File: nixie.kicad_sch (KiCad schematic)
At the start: 28 parts, among them IC1 SN74141, IC2 SN74141, IC3 SN74141, IC4 SN74141, IC5 MIC5219-5.0YM5-TR, IC6 DS3231M+TRL, J1 1984989

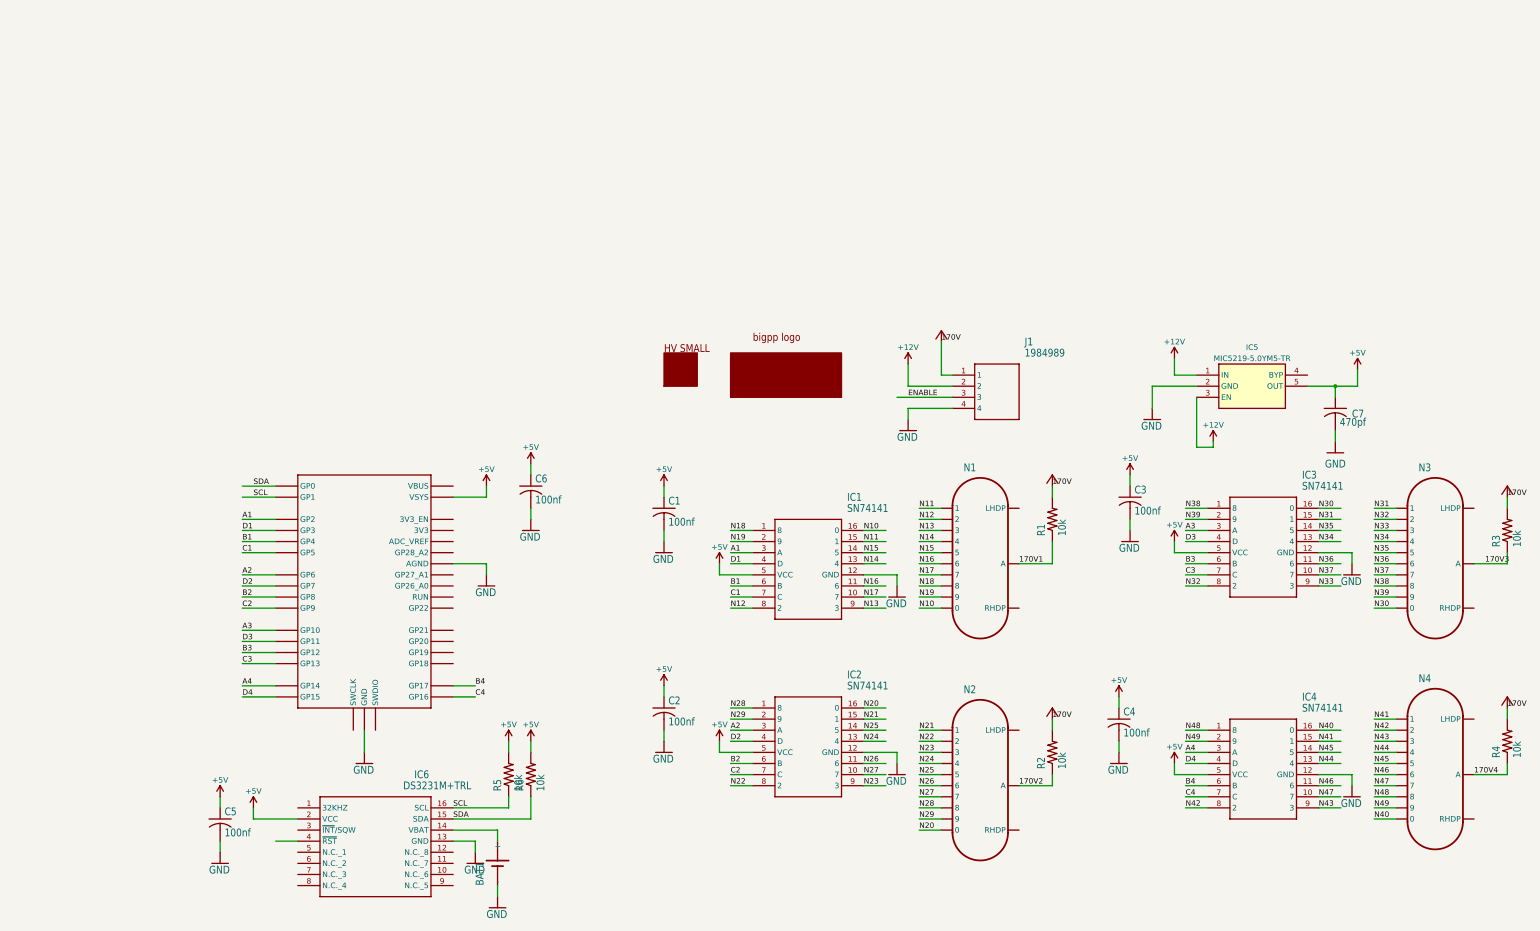
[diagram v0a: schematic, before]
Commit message: Adding WIP files
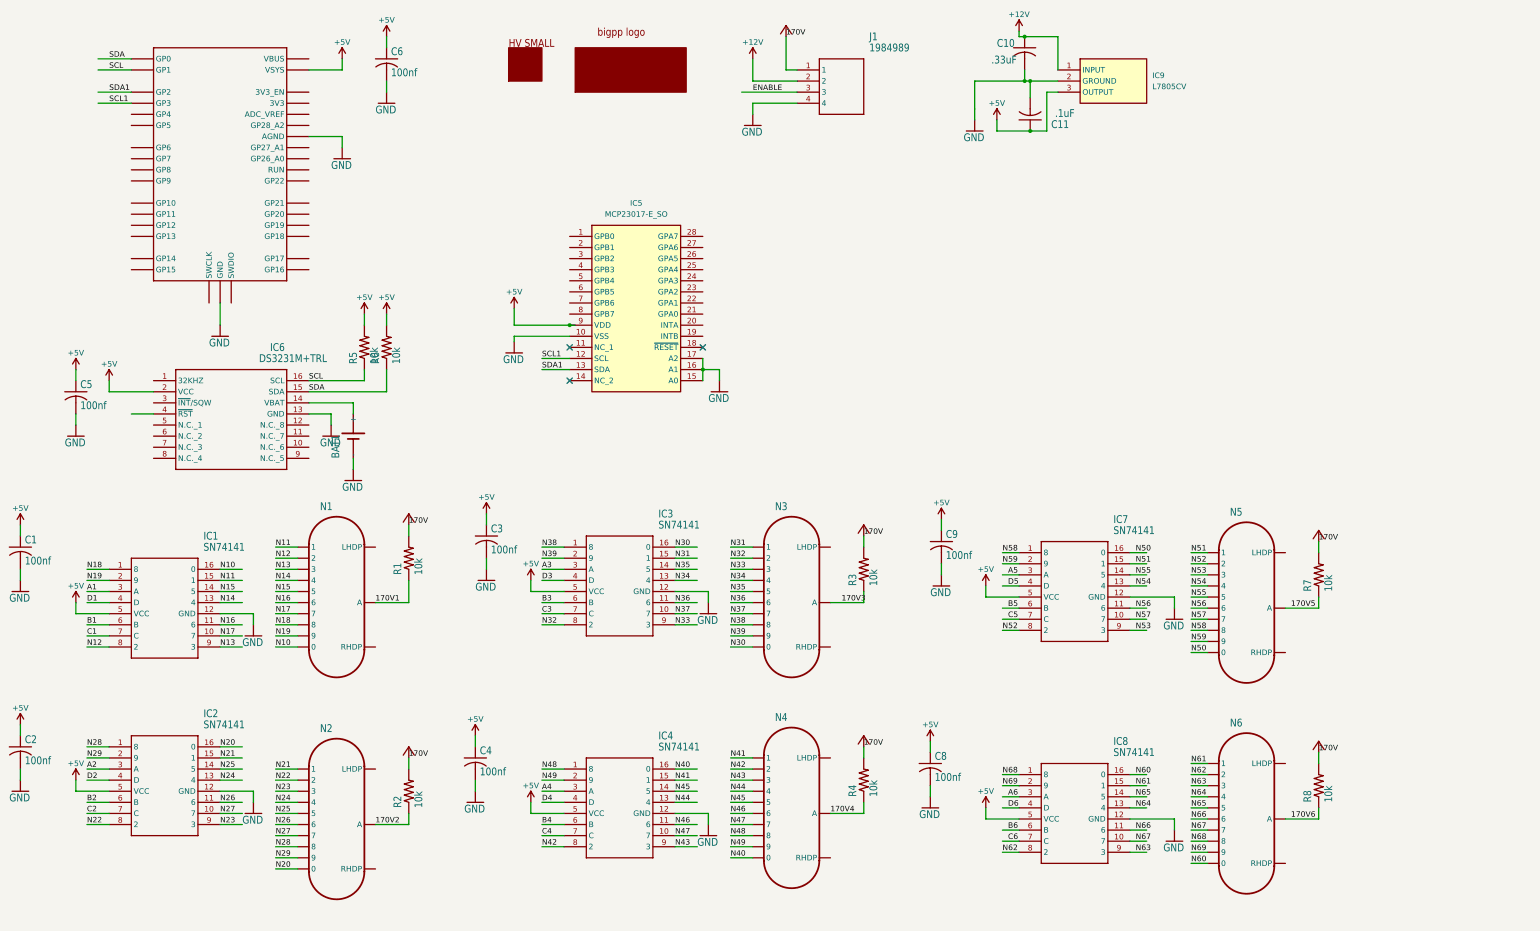
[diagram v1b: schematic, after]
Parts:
- removed C7: 470pf, nixie:C0805, symbol nixie-eagle-import:C-USC0805
- removed IC5: MIC5219-5.0YM5-TR, SOT95P280X130-5N, symbol MIC5219-5_0YM5-TR:MIC5219-5.0YM5-TR
- added C10: .33uF, nixie:C0805, symbol nixie-eagle-import:C-USC0805
- added C11: .1uF, nixie:C0805, symbol nixie-eagle-import:C-USC0805
- added C8, C9: 100nf, nixie:C0805, symbol nixie-eagle-import:C-USC0805
- added IC5: MCP23017-E_SO, L7805CV:SOIC127P1030X265-28N, symbol MCP23017-E_SO:MCP23017-E_SO
- added IC7, IC8: SN74141, TimeExpander:DIP16-2.54-19.2X7.62MM, symbol nixie-eagle-import:SN74141
- added IC9: L7805CV, L7805CV:TO255P460X1020X2008-3P, symbol L7805CV:L7805CV
- added N5, N6: IN-14, nixie:IN-14, symbol nixie-eagle-import:IN-14
- added R7, R8: 10k, nixie:R0805, symbol nixie-eagle-import:R-US_R0805
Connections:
- net +12V: now also C10.1, IC9.1 (INPUT)
- net +5V: now also C11.1, C8.1, C9.1, IC5.9 (VDD), IC7.5 (VCC), IC8.5 (VCC), IC9.3 (OUTPUT)
- net A1: no longer U$1.GP2
- net A2: no longer U$1.GP6
- net A3: no longer U$1.GP10
- net A4: no longer U$1.GP14
- net B1: no longer U$1.GP4
- net B2: no longer U$1.GP8
- net B3: no longer U$1.GP12
- net B4: no longer U$1.GP17
- net C1: no longer U$1.GP5
- net C2: no longer U$1.GP9
- net C3: no longer U$1.GP13
- net C4: no longer U$1.GP16
- net D1: no longer U$1.GP3
- net D2: no longer U$1.GP7
- net D3: no longer U$1.GP11
- net D4: no longer U$1.GP15
- net GND: now also C10.2, C11.2, C8.2, C9.2, IC5.10 (VSS), IC5.15 (A0), IC5.16 (A1), IC5.17 (A2), IC7.12 (GND), IC8.12 (GND), IC9.2 (GROUND)
- net VCC: now also R7.2, R8.2
- new net 170V5: N5.A, R7.1
- new net 170V6: N6.A, R8.1
- new net A5: IC7.3 (A)
- new net A6: IC8.3 (A)
- new net B5: IC7.6 (B)
- new net B6: IC8.6 (B)
- new net C5: IC7.7 (C)
- new net C6: IC8.7 (C)
- new net D5: IC7.4 (D)
- new net D6: IC8.4 (D)
- new net N50: IC7.16 (0), N5.0
- new net N51: IC7.15 (1), N5.1
- new net N52: IC7.8 (2), N5.2
- new net N53: IC7.9 (3), N5.3
- new net N54: IC7.13 (4), N5.4
- new net N55: IC7.14 (5), N5.5
- new net N56: IC7.11 (6), N5.6
- new net N57: IC7.10 (7), N5.7
- new net N58: IC7.1 (8), N5.8
- new net N59: IC7.2 (9), N5.9
- new net N60: IC8.16 (0), N6.0
- new net N61: IC8.15 (1), N6.1
- new net N62: IC8.8 (2), N6.2
- new net N63: IC8.9 (3), N6.3
- new net N64: IC8.13 (4), N6.4
- new net N65: IC8.14 (5), N6.5
- new net N66: IC8.11 (6), N6.6
- new net N67: IC8.10 (7), N6.7
- new net N68: IC8.1 (8), N6.8
- new net N69: IC8.2 (9), N6.9
- new net SCL1: IC5.12 (SCL), U$1.GP3
- new net SDA1: IC5.13 (SDA), U$1.GP2
- no-connect marks 0 -> 3
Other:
- moved on the sheet: BAT1, C1, C2, C3, C4, C5, C6, IC1, IC2, IC3, IC4, IC6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

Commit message: revert
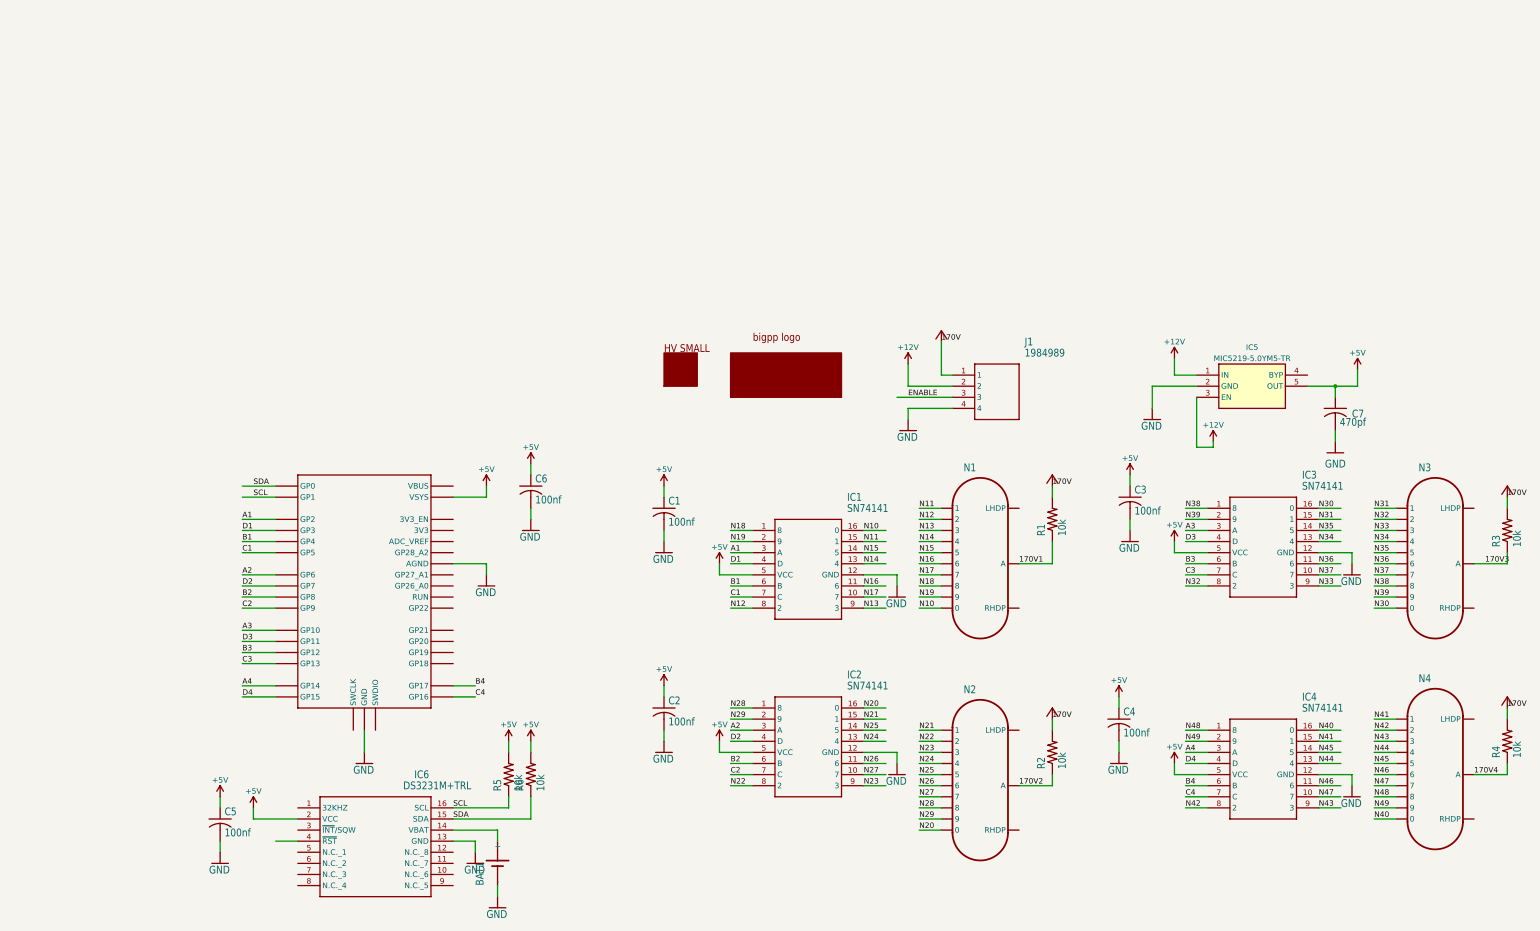
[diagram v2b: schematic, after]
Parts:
- removed C10: .33uF, nixie:C0805, symbol nixie-eagle-import:C-USC0805
- removed C11: .1uF, nixie:C0805, symbol nixie-eagle-import:C-USC0805
- removed C8, C9: 100nf, nixie:C0805, symbol nixie-eagle-import:C-USC0805
- removed IC5: MCP23017-E_SO, L7805CV:SOIC127P1030X265-28N, symbol MCP23017-E_SO:MCP23017-E_SO
- removed IC7, IC8: SN74141, TimeExpander:DIP16-2.54-19.2X7.62MM, symbol nixie-eagle-import:SN74141
- removed IC9: L7805CV, L7805CV:TO255P460X1020X2008-3P, symbol L7805CV:L7805CV
- removed N5, N6: IN-14, nixie:IN-14, symbol nixie-eagle-import:IN-14
- removed R7, R8: 10k, nixie:R0805, symbol nixie-eagle-import:R-US_R0805
- added C7: 470pf, nixie:C0805, symbol nixie-eagle-import:C-USC0805
- added IC5: MIC5219-5.0YM5-TR, SOT95P280X130-5N, symbol MIC5219-5_0YM5-TR:MIC5219-5.0YM5-TR
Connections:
- net SCL1 is gone; now on net D1: U$1.GP3
- net SDA1 is gone; now on net A1: U$1.GP2
- net +12V: now also IC5.1 (IN), IC5.3 (EN)
- net +5V: now also C7.1, IC5.5 (OUT)
- net A2: now also U$1.GP6
- net A3: now also U$1.GP10
- net A4: now also U$1.GP14
- net B1: now also U$1.GP4
- net B2: now also U$1.GP8
- net B3: now also U$1.GP12
- net B4: now also U$1.GP17
- net C1: now also U$1.GP5
- net C2: now also U$1.GP9
- net C3: now also U$1.GP13
- net C4: now also U$1.GP16
- net D2: now also U$1.GP7
- net D3: now also U$1.GP11
- net D4: now also U$1.GP15
- net GND: now also C7.2, IC5.2 (GND)
- no-connect marks 3 -> 0
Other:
- moved on the sheet: BAT1, C1, C2, C3, C4, C5, C6, IC1, IC2, IC3, IC4, IC6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
